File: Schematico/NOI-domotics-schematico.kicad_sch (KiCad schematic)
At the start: 40 parts

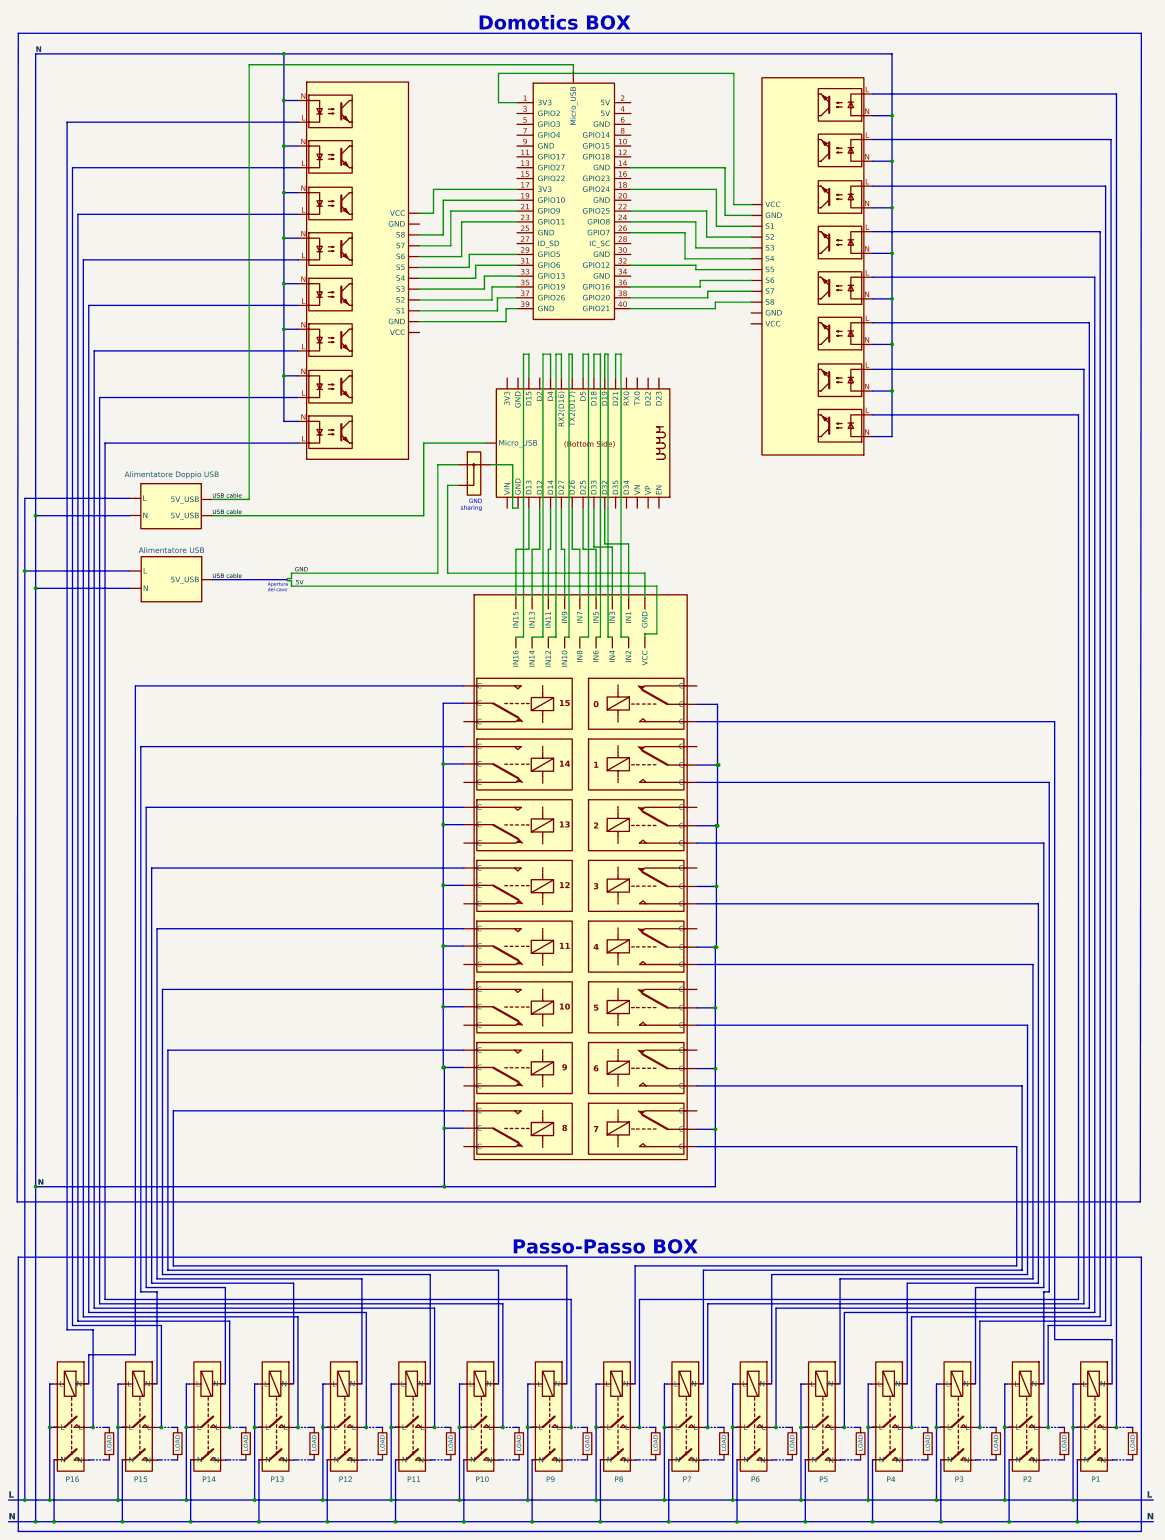
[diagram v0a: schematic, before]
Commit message: schehge
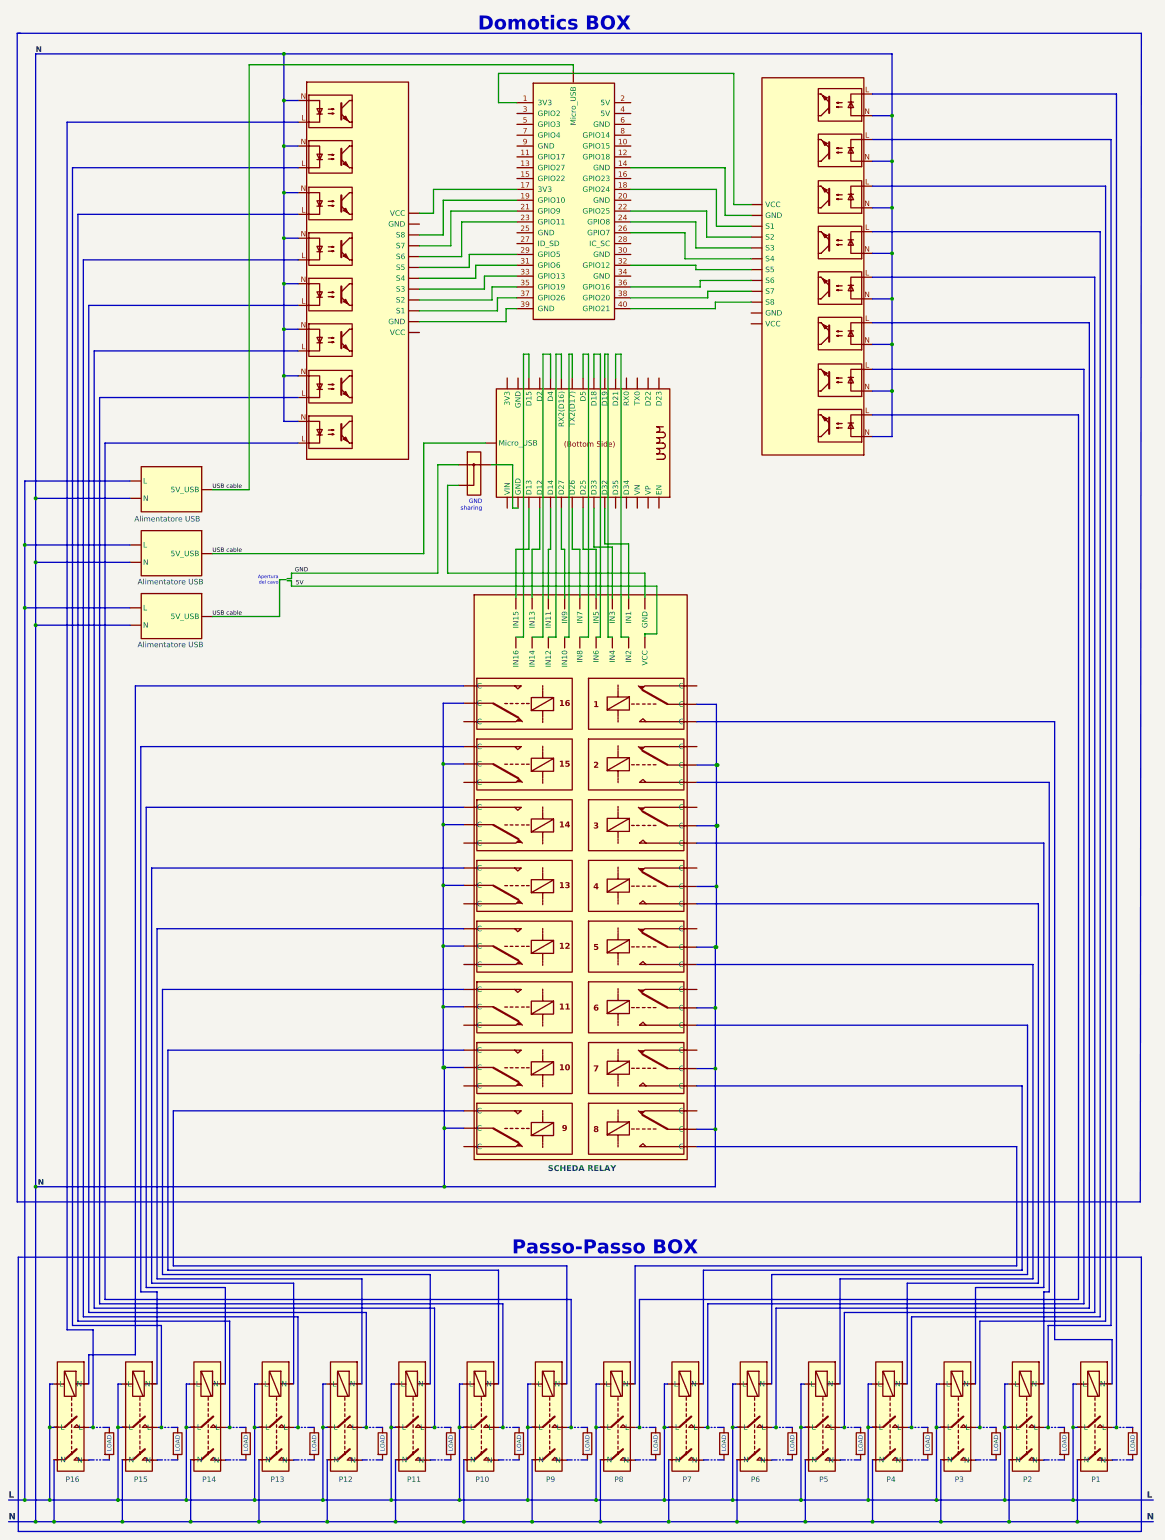
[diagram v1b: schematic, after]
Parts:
- removed U?: Alimentatore Doppio USB, symbol USB_5V:USB_DCconverter
- added U? (x2): Alimentatore USB, symbol USB_5V:USB_DCconverter
- K?: value (none) -> SCHEDA RELAY
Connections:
- net USB cable: now also U?. (N), U?. (N)
- net at U?. (VCC): now also J?.39 (GND)
- net at U?.1 (VP): no longer RN?.
- new net: K?. (VCC), RN?.
- new net: RN?., U?.1 (VP)
- new net: K?. (VCC), U?.1 (VP) (x16)
- now unconnected: U?.1 (VP), U?.1 (VP), U?.1 (VP), U?.1 (VP), U?.1 (VP), U?.1 (VP), U?.1 (VP), U?.1 (VP), U?.1 (VP), U?.1 (VP), U?.1 (VP), U?.1 (VP), U?.1 (VP), U?.1 (VP), U?.1 (VP), U?.1 (VP)
